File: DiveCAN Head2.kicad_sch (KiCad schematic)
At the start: 73 parts, among them J1 C1, J2 C2, J3 C3, J4 AUX, J5 Solenoid, J7 CAN, Q1 DMG1012T, U1 ADS1115IDGS, U2 ADS1115IDGS, U5 STM32L431RCTx, U6 TCAN33X, Y1 8MHz

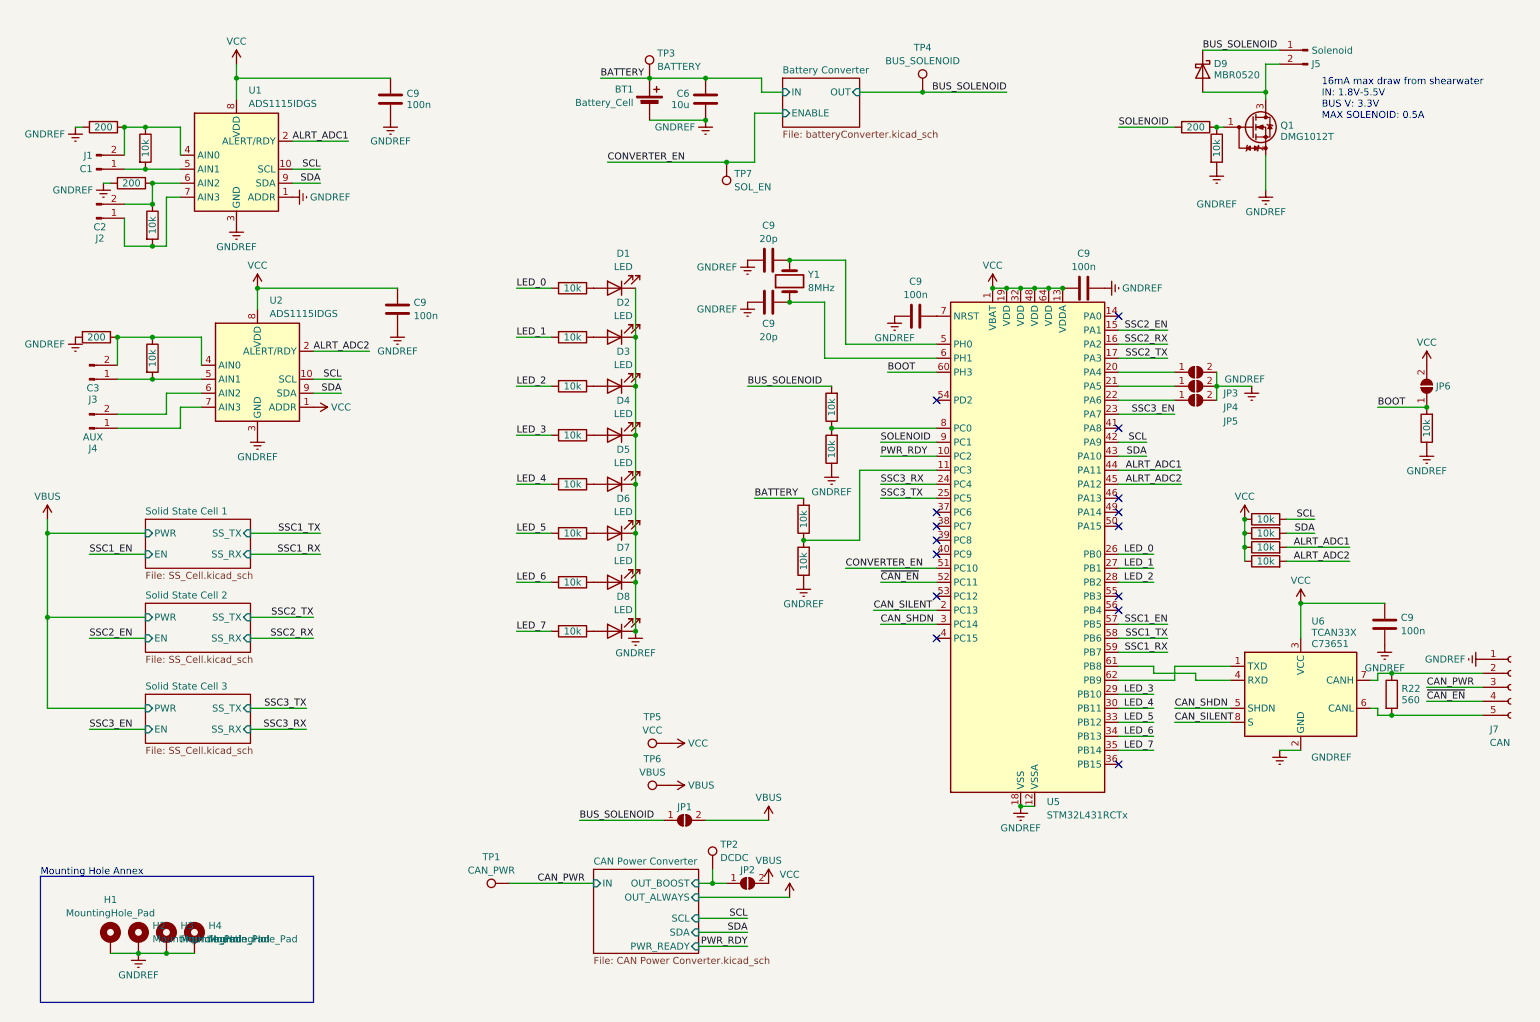
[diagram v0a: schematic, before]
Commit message: Revision 2.1 HW
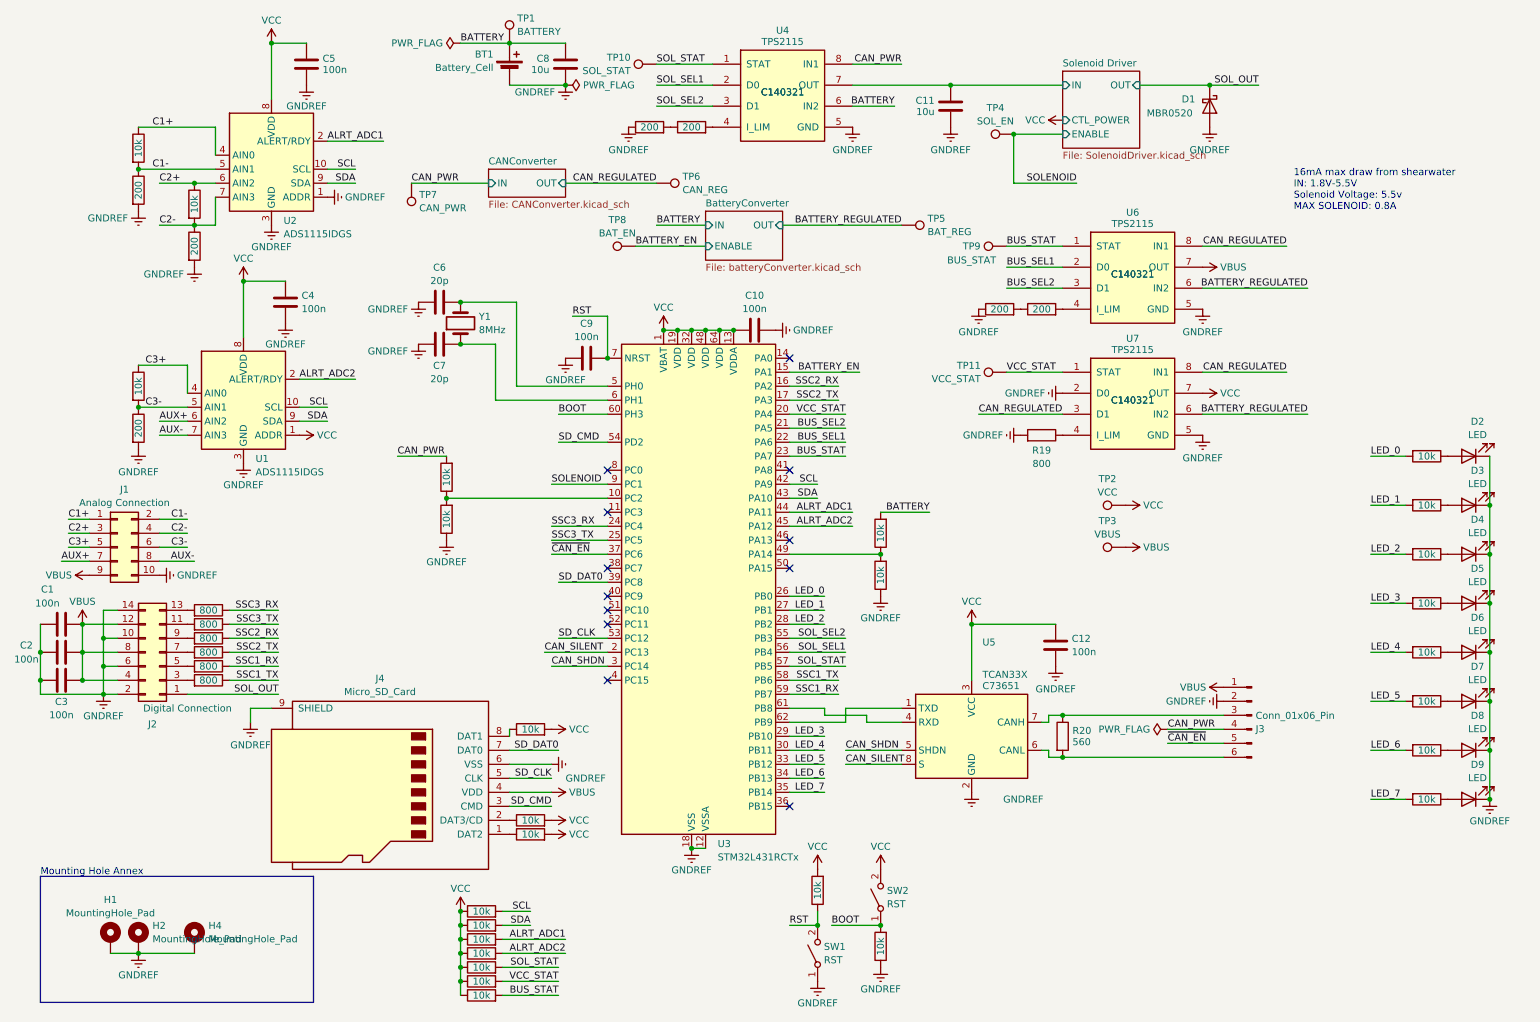
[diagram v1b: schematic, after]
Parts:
- removed C6: 10u, Capacitor_SMD:C_0603_1608Metric, symbol Library:C
- removed H3: MountingHole_Pad, MountingHole:MountingHole_2.2mm_M2_Pad, symbol Library:MountingHole_Pad
- removed J1: C1, Connector_JST:JST_SH_BM02B-SRSS-TB_1x02-1MP_P1.00mm_Vertical, symbol Library:Conn_01x02_Pin
- removed J2: C2, Connector_JST:JST_SH_BM02B-SRSS-TB_1x02-1MP_P1.00mm_Vertical, symbol Library:Conn_01x02_Pin
- removed J3: C3, Connector_JST:JST_SH_BM02B-SRSS-TB_1x02-1MP_P1.00mm_Vertical, symbol Library:Conn_01x02_Pin
- removed J4: AUX, Connector_JST:JST_SH_BM02B-SRSS-TB_1x02-1MP_P1.00mm_Vertical, symbol Library:Conn_01x02_Pin
- removed J5: Solenoid, Connector_JST:JST_SH_BM02B-SRSS-TB_1x02-1MP_P1.00mm_Vertical, symbol Library:Conn_01x02_Pin
- removed J7: CAN, TerminalBlock_Phoenix:TerminalBlock_Phoenix_MPT-0,5-5-2.54_1x05_P2.54mm_Horizontal, symbol Library:Conn_01x05_Socket
- removed JP1, JP2, JP3, JP4, JP5, JP6: ~, Jumper:SolderJumper-2_P1.3mm_Open_Pad1.0x1.5mm, symbol Library:SolderJumper_2_Open
- removed Q1: DMG1012T, Package_TO_SOT_SMD:SOT-523, symbol Library:DMG1012T
- removed R20, R34, R35, R36: 200, Resistor_SMD:R_0402_1005Metric, symbol Library:R
- removed R21, R32, R33: 10k, Resistor_SMD:R_0402_1005Metric, symbol Library:R
- removed TP2: DCDC, TestPoint:TestPoint_THTPad_D1.0mm_Drill0.5mm, symbol Library:TestPoint
- removed TP3: BATTERY, TestPoint:TestPoint_THTPad_D1.0mm_Drill0.5mm, symbol Library:TestPoint
- removed TP4: BUS_SOLENOID, TestPoint:TestPoint_THTPad_D1.0mm_Drill0.5mm, symbol Library:TestPoint
- added C1, C2, C3: 100n, Capacitor_SMD:C_0603_1608Metric, symbol Library:C
- added C11, C8: 10u, Capacitor_SMD:C_0603_1608Metric, symbol Library:C
- added J1: Analog Connection, Connector_IDC:IDC-Header_2x05_P2.54mm_Vertical, symbol Connector_Generic:Conn_02x05_Odd_Even
- added J2: Digital Connection, Connector_IDC:IDC-Header_2x07_P2.54mm_Vertical, symbol Connector_Generic:Conn_02x07_Odd_Even
- added J3: Conn_01x06_Pin, TerminalBlock_Phoenix:TerminalBlock_Phoenix_MPT-0,5-6-2.54_1x06_P2.54mm_Horizontal, symbol Connector:Conn_01x06_Pin
- added J4: Micro_SD_Card, Library:CONN9_0185-02_GSW, symbol Connector:Micro_SD_Card
- added R11, R12, R16, R18, R40, R41, R43, R45, R46, R47: 10k, Resistor_SMD:R_0402_1005Metric, symbol Library:R
- added R15, R2, R4, R42, R44, R6: 200, Resistor_SMD:R_0402_1005Metric, symbol Library:R
- added R19, R48, R49, R50, R51, R52, R53: 800, Resistor_SMD:R_0402_1005Metric, symbol Project:R
- added SW1, SW2: RST, Button_Switch_SMD:SW_SPST_EVQPE1, symbol Switch:SW_SPST
- added TP10: SOL_STAT, TestPoint:TestPoint_THTPad_D1.0mm_Drill0.5mm, symbol Library:TestPoint
- added TP11: VCC_STAT, TestPoint:TestPoint_THTPad_D1.0mm_Drill0.5mm, symbol Library:TestPoint
- added TP5: BAT_REG, TestPoint:TestPoint_THTPad_D1.0mm_Drill0.5mm, symbol Library:TestPoint
- added TP6: CAN_REG, TestPoint:TestPoint_THTPad_D1.0mm_Drill0.5mm, symbol Library:TestPoint
- added TP7: CAN_PWR, TestPoint:TestPoint_THTPad_D1.0mm_Drill0.5mm, symbol Library:TestPoint
- added TP8: BAT_EN, TestPoint:TestPoint_THTPad_D1.0mm_Drill0.5mm, symbol Library:TestPoint
- added TP9: BUS_STAT, TestPoint:TestPoint_THTPad_D1.0mm_Drill0.5mm, symbol Library:TestPoint
- added U4, U6, U7: TPS2115, Library:VSON-8_3.3x3.3mm_P0.65mm_NexFET, symbol Project:TPS2115
- BT1: JLC C5290176 -> C5290175
- H1, H2, H4: footprint MountingHole:MountingHole_2.2mm_M2_Pad -> MountingHole:MountingHole_3.2mm_M3_Pad
- R14: value 10k -> 200; MPN C26083 -> C25087
- TP1: value CAN_PWR -> BATTERY
- renumbered C9 to C10, C9 to C12, C9 to C4, C9 to C5, C9 to C6, C9 to C7, D9 to D1, D1 to D2, D2 to D3, D3 to D4, D4 to D5, D5 to D6, D6 to D7, D7 to D8, D8 to D9, R31 to R1, R19 to R10, R15 to R17, R22 to R20, R1 to R21, R2 to R22, R3 to R23, R4 to R24, R5 to R25, R6 to R26, R7 to R27, R8 to R28, R29 to R3, R30 to R5, R16 to R7, R17 to R8, R18 to R9, TP5 to TP2, TP6 to TP3, TP7 to TP4, U2 to U1, U1 to U2, U5 to U3, U6 to U5
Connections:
- net BATTERY: now also TP1.1, C8.2, R12.2, U4.6 (IN2)
- net BOOT: now also SW2.1 (A)
- net CAN_PWR: now also J3.4 (Pin_4), R46.2, TP7.1, U4.8 (IN1); no longer TP1.1
- net GNDREF: now also D1.2 (A), R13.1, C1.1, C11.1, C2.1, C3.1, C8.1, J1.10 (Pin_10), J2.10 (Pin_10), J2.14 (Pin_14), J2.2 (Pin_2), J2.6 (Pin_6), J3.2 (Pin_2), J4.6 (VSS), J4.9 (SHIELD), R19.2, R2.2, R4.2, R42.1, R47.1, R6.2, SW1.1 (A), U4.5 (GND), U6.5 (GND), U7.2 (D0), U7.5 (GND)
- net SOLENOID: now also TP4.1
- net SSC1_RX: now also R52.1
- net SSC1_TX: now also R53.1
- net SSC2_RX: now also R50.1
- net SSC2_TX: now also R51.1
- net SSC3_RX: now also R48.1
- net SSC3_TX: now also R49.1
- net VBUS: now also C1.2, C2.2, C3.2, J1.9 (Pin_9), J2.12 (Pin_12), J2.4 (Pin_4), J2.8 (Pin_8), J3.1 (Pin_1), J4.4 (VDD), U6.7 (OUT)
- net VCC: now also R11.1, R16.2, R18.1, R40.2, R41.2, R43.2, R45.1, SW2.2 (B), U7.7 (OUT)
- net ~{CAN_EN}: now also U3.37 (PC6), J3.5 (Pin_5); no longer U3.52 (PC11)
- net at R20.1, U5.7 (CANH): now also J3.3 (Pin_3)
- net at R20.2, U5.6 (CANL): now also J3.6 (Pin_6)
- net VCC_STAT: now reaches U3.20 (PA4)
- net VCC_STAT: now also R18.2, TP11.1, U7.1 (STAT)
- net C3+: now reaches R3.1, U1.4 (AIN0)
- net C3+: now also J1.5 (Pin_5)
- net C3-: now reaches R3.2, U1.5 (AIN1)
- net C3-: now also J1.6 (Pin_6), R4.1
- net BUS_SEL1: now reaches U3.22 (PA6)
- net BUS_SEL1: now also U6.2 (D0)
- net C1+: now reaches R1.1, U2.4 (AIN0)
- net C1+: now also J1.1 (Pin_1)
- net C1-: now reaches R1.2, U2.5 (AIN1)
- net C1-: now also J1.2 (Pin_2), R2.1
- net C2+: now reaches R5.1, U2.6 (AIN2)
- net C2+: now also J1.3 (Pin_3)
- net C2-: now reaches R5.2, U2.7 (AIN3)
- net C2-: now also J1.4 (Pin_4), R6.1
- net RST: now reaches C9.2, U3.7 (NRST)
- net RST: now also R16.1, SW1.2 (B)
- net AUX+: now reaches U1.6 (AIN2)
- net AUX+: now also J1.7 (Pin_7)
- net AUX-: now reaches U1.7 (AIN3)
- net AUX-: now also J1.8 (Pin_8)
- net BUS_SEL2: now reaches U3.21 (PA5)
- net BUS_SEL2: now also U6.3 (D1)
- net SD_DAT0: now reaches U3.39 (PC8)
- net SD_DAT0: now also J4.7 (DAT0)
- net at U3.49 (PA14): now also R13.2, R12.1
- net SD_CLK: now reaches U3.53 (PC12)
- net SD_CLK: now also J4.5 (CLK)
- net SD_CMD: now reaches U3.54 (PD2)
- net SD_CMD: now also J4.3 (CMD)
- net SOL_SEL2: now reaches U3.55 (PB3)
- net SOL_SEL2: now also U4.3 (D1)
- net SOL_SEL1: now reaches U3.56 (PB4)
- net SOL_SEL1: now also U4.2 (D0)
- net BUS_SOLENOID renamed SOL_OUT
- net SOL_OUT: now also J2.1 (Pin_1); no longer R13.2
- net CONVERTER_EN: no longer names the net of U3.51 (PC10)
- net CONVERTER_EN: no longer TP4.1
- net PWR_RDY: no longer names the net of U3.10 (PC2)
- net PWR_RDY: now also R46.1, R47.2
- net SSC1_EN renamed SOL_STAT
- net SOL_STAT: now also R11.2, TP10.1, U4.1 (STAT)
- net SSC2_EN renamed BATTERY_EN
- net BATTERY_EN: now also TP8.1
- net SSC3_EN renamed BUS_STAT
- net BUS_STAT: now also R45.2, TP9.1, U6.1 (STAT)
- new net: R42.2, R44.1
- new net: R44.2, U6.4 (I_LIM)
- new net: R19.1, U7.4 (I_LIM)
- new net: J2.7 (Pin_7), R51.2
- new net: J4.2 (DAT3/CD), R41.1
- new net: J2.11 (Pin_11), R49.2
- new net: J2.9 (Pin_9), R50.2
- new net: J2.5 (Pin_5), R52.2
- new net: J4.1 (DAT2), R40.1
- new net: J4.8 (DAT1), R43.1
- new net: R14.2, R15.1
- new net: R15.2, U4.4 (I_LIM)
- new net: J2.13 (Pin_13), R48.2
- new net: J2.3 (Pin_3), R53.2
- new net BATTERY_REGULATED: TP5.1, U6.6 (IN2), U7.6 (IN2)
- new net CAN_REGULATED: TP6.1, U6.8 (IN1), U7.3 (D1), U7.8 (IN1)
- new net Solenoid Driver/IN: C11.2, U4.7 (OUT)
- now unconnected: U3.8 (PC0)
- no-connect marks 15 -> 12
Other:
- sheet Battery Converter renamed Solenoid Driver
- removed sheet CAN Power Converter
- removed sheet Solid State Cell 1
- removed sheet Solid State Cell 2
- removed sheet Solid State Cell 3
- added sheet BatteryConverter (batteryConverter.kicad_sch)
- added sheet CANConverter (CANConverter.kicad_sch)
- sheet Solenoid Driver: file batteryConverter.kicad_sch -> SolenoidDriver.kicad_sch
- sheet Solenoid Driver ports: added CTL_POWER; removed none
- note added: "16mA max draw from shearwater IN: 1.8V-5.5V Solenoid Voltage: 5.5v MAX SOLENOID: 0.8A"
- note removed: "16mA max draw from shearwater IN: 1.8V-5.5V BUS V: 3.3V MAX SOLENOID: 0.5A"
- moved on the sheet: C10, C12, C4, C5, C6, C7, C9, D1, D2, D3, D4, D5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
